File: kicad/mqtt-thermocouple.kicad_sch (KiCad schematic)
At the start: 24 parts, among them J1 Barrel_Jack, Q1 2N7000, Q2 2N7000, U1 MCP9600-E_MX, U2 CD4060BM96

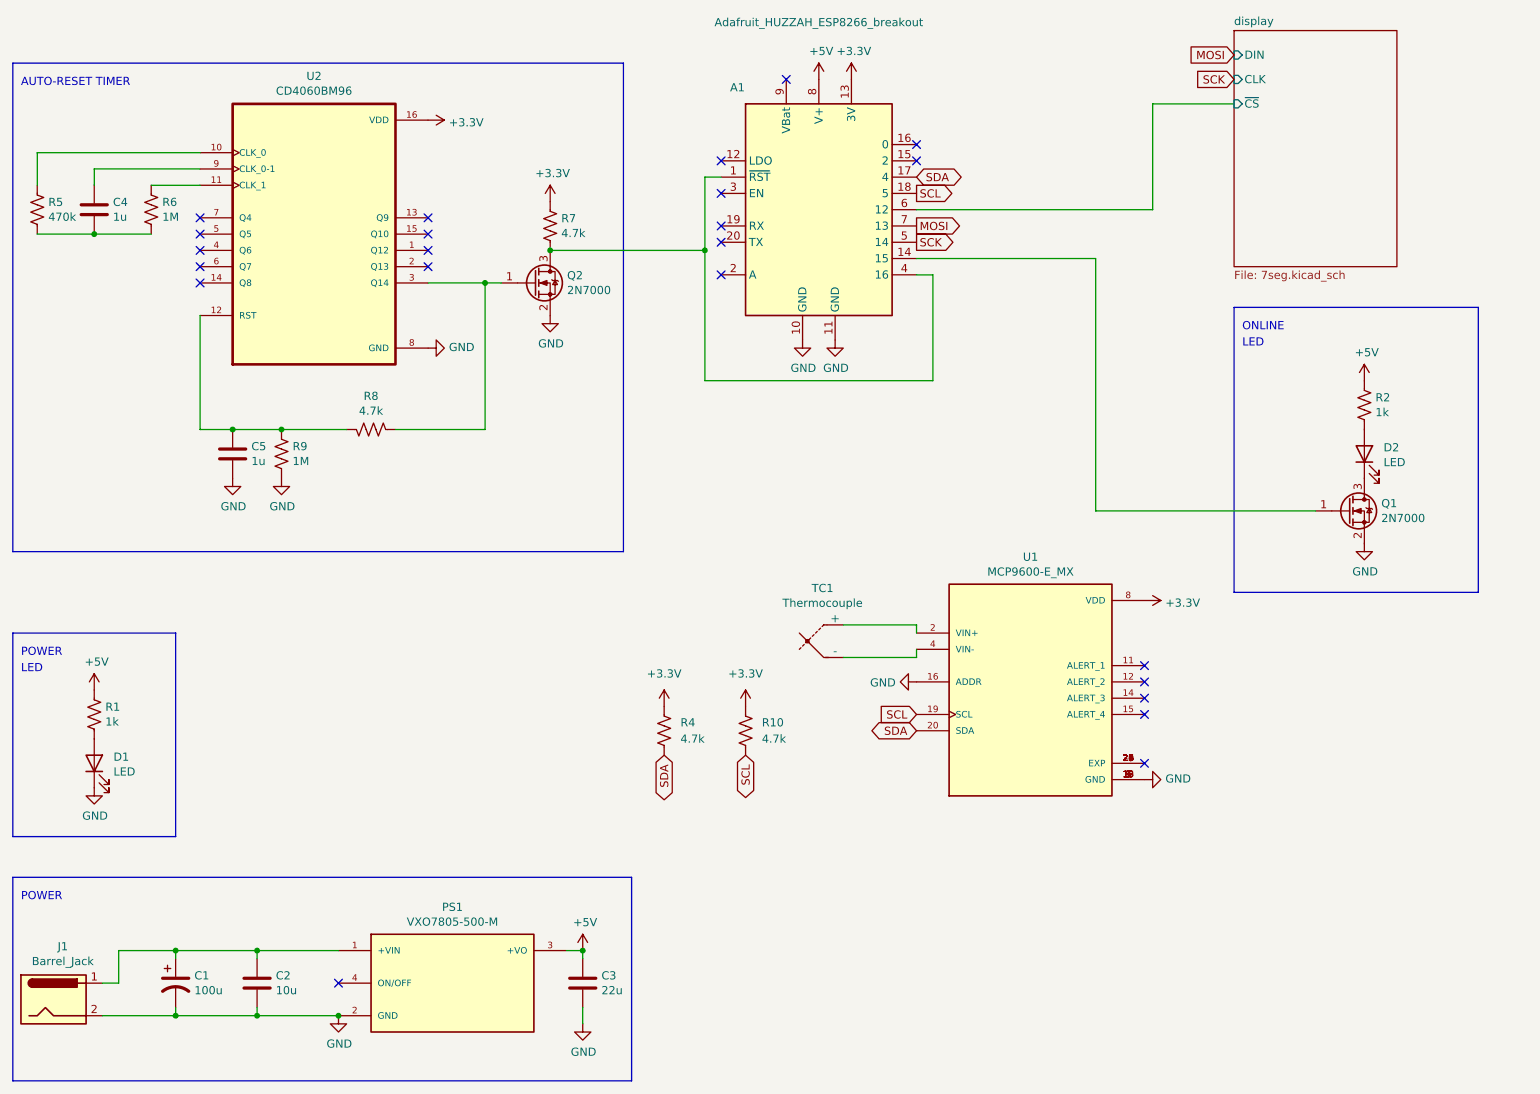
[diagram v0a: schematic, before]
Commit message: checkpoint
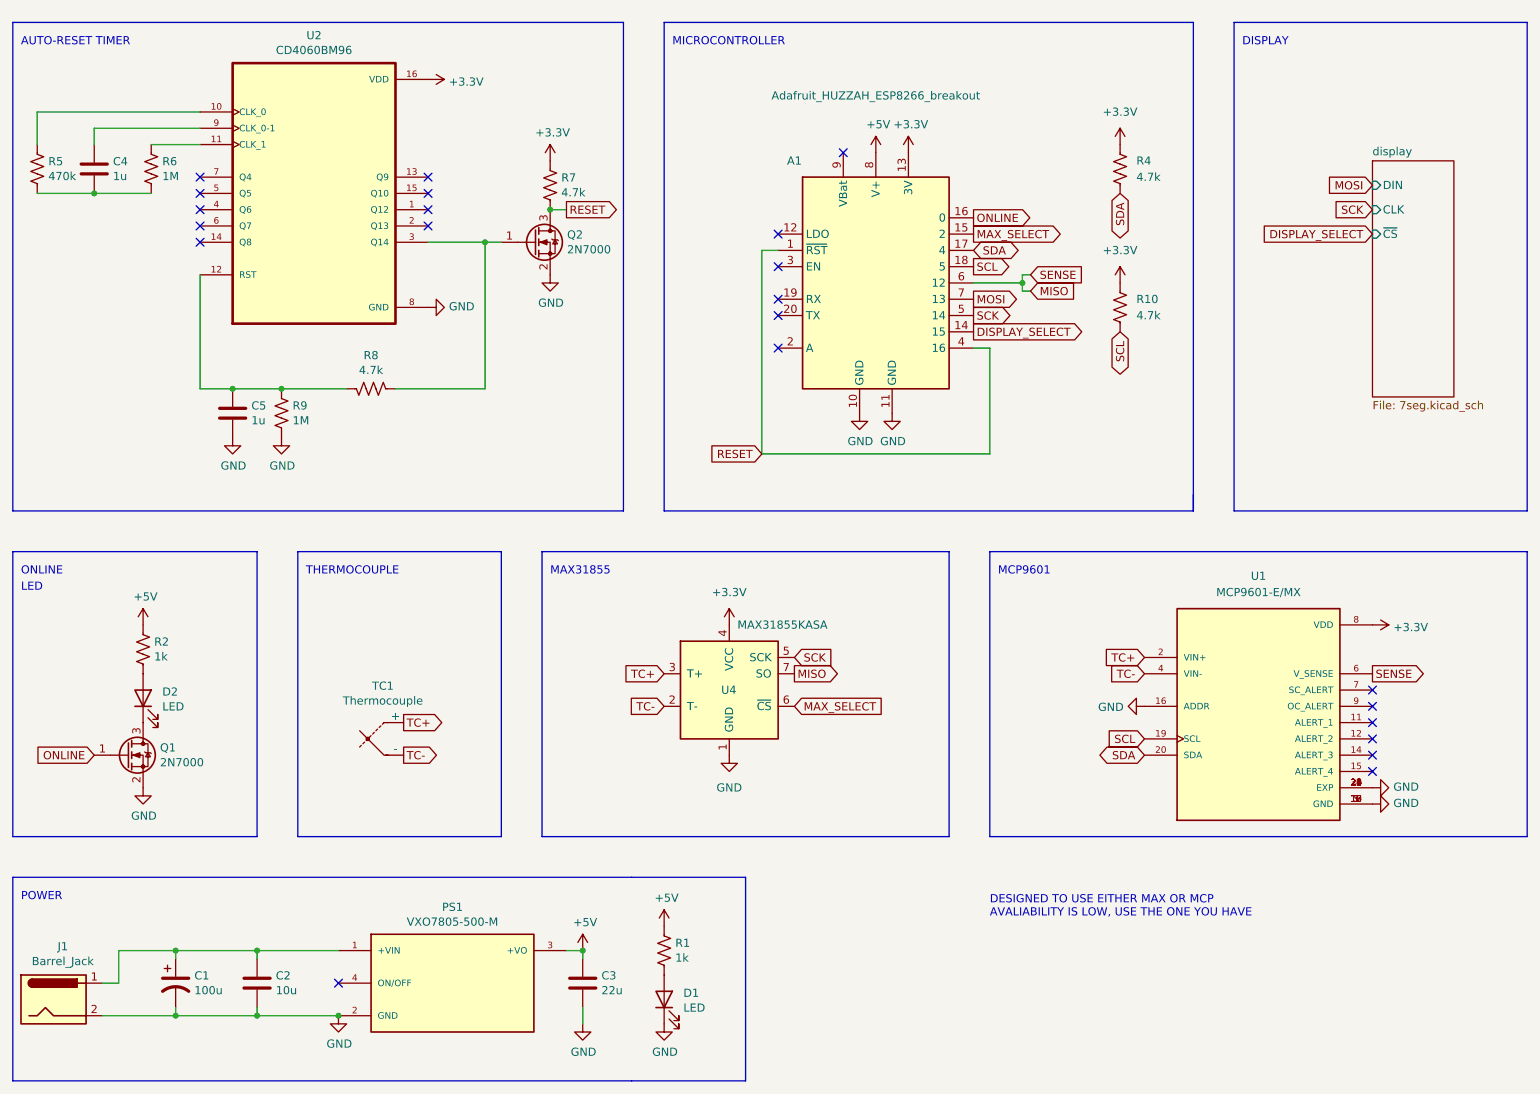
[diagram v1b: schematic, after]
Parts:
- removed U1: MCP9600-E_MX, footprints:MX, symbol MCP9600-E_MX:MCP9600-E_MX
- added U1: MCP9601-E/MX, QFN65P500X500X100-21N_MCP9600-E/MX, symbol MCP9601-E_MX:MCP9601-E/MX
- added U4: MAX31855KASA, Package_SO:SOIC-8_3.9x4.9mm_P1.27mm, symbol Sensor_Temperature:MAX31855KASA
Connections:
- net +3V3: now also U1.8 (VDD)
- net GND: now also U1.1 (GND), U1.10 (GND), U1.13 (GND), U1.16 (ADDR), U1.17 (GND), U1.18 (GND), U1.21 (EXP), U1.22 (EXP), U1.23 (EXP), U1.24 (EXP), U1.25 (EXP), U1.26 (EXP), U1.27 (EXP), U1.28 (EXP), U1.29 (EXP), U1.3 (GND), U1.30 (EXP), U1.5 (GND), U4.1 (GND)
- net SCK: now also U4.5 (SCK)
- net SCL: now also U1.19 (SCL)
- net SDA: now also U1.20 (SDA)
- net RESET: now reaches A1.1 (~{RST}), A1.4 (16), Q2.3 (D), R7.2
- net DISPLAY_SELECT: now reaches A1.14 (15)
- net DISPLAY_SELECT: no longer Q1.1 (G)
- net MAX_SELECT: now reaches A1.15 (2)
- net MAX_SELECT: now also U4.6 (~{CS})
- net ONLINE: now reaches A1.16 (0)
- net ONLINE: now also Q1.1 (G)
- net TC+: now reaches TC1.1 (+)
- net TC+: now also U1.2 (VIN+), U4.3 (T+)
- net TC-: now reaches TC1.2 (-)
- net TC-: now also U1.4 (VIN-), U4.2 (T-)
- net display/~{CS} renamed MISO
- net MISO: now also U1.6 (V_SENSE), U4.7 (SO)
- new net +3.3V: U4.4 (VCC)
- no-connect marks 23 -> 22
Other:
- note added: "DESIGNED TO USE EITHER MAX OR MCP AVALIABILITY IS LOW, USE THE ONE YOU HAVE"
- note added: "DISPLAY"
- note added: "MAX31855"
- note added: "MCP9601"
- note added: "MICROCONTROLLER"
- note added: "THERMOCOUPLE"
- moved on the sheet: A1, C4, C5, D1, D2, Q1, Q2, R1, R10, R2, R4, R5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
